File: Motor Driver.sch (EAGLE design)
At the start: 25 parts, among them U1 DRV8432_DKD_36, U2 LM27313

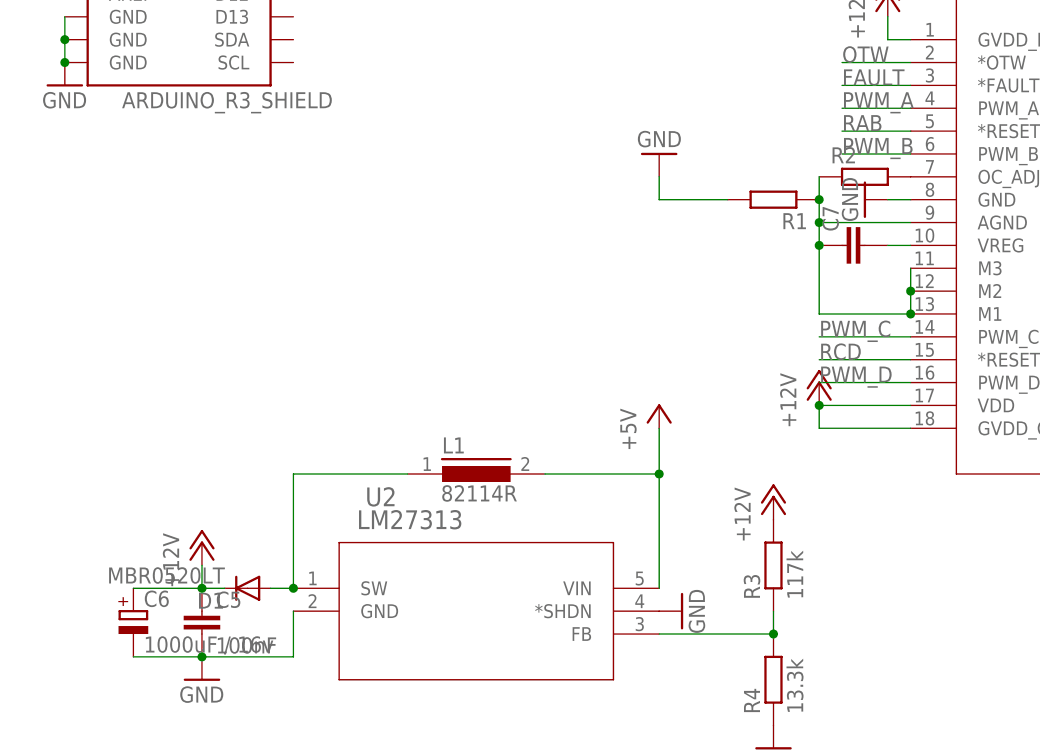
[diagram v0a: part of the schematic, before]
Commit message: Uploading Board
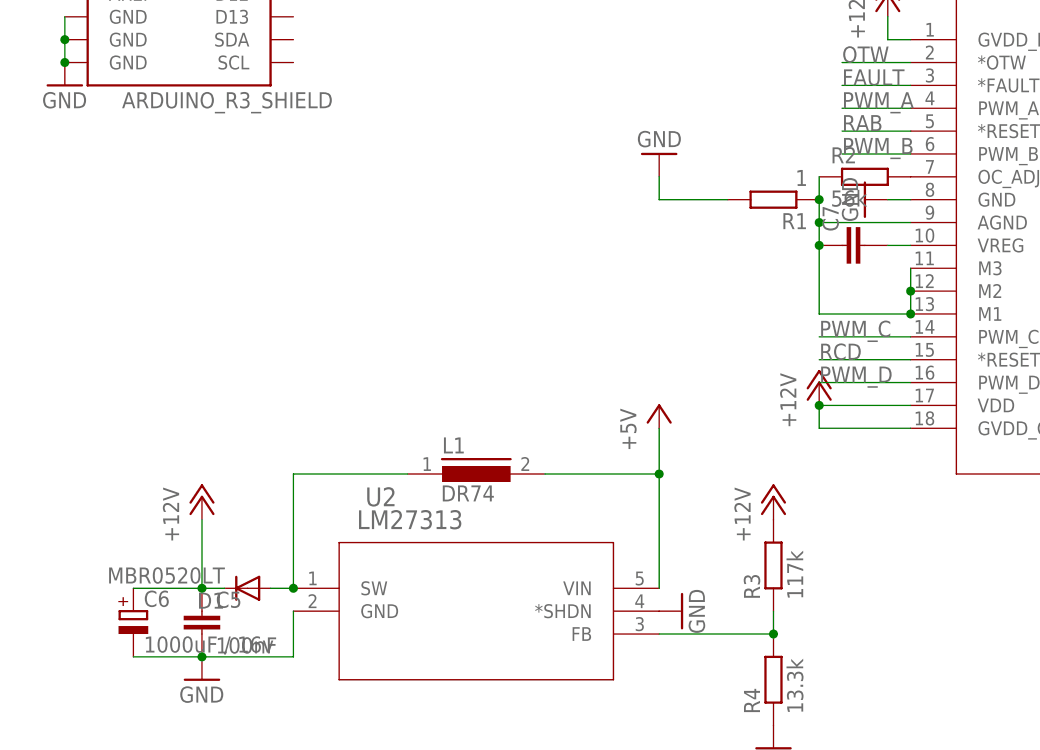
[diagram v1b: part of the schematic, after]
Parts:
- C1, C2, C3, C4: device resistor:C-EUC0805K -> resistor:C-EUC0402K
- L1: value 82114R -> DR74; device inductors:82114R -> inductors:DR74
- R1: value (none) -> 1
- R2: value (none) -> 56k
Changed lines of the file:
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@@
 <part name="U2" library="LM27313" deviceset="LM27313" device=""/>
 <part name="P+9" library="supply1" deviceset="+5V" device=""/>
-<part name="L1" library="inductors" deviceset="82114R" device=""/>
+<part name="L1" library="inductors" deviceset="DR74" device=""/>
 <part name="D1" library="diode" deviceset="MBR0520LT" device=""/>
 <part name="C5" library="resistor" deviceset="C-EU" device="C0805K" value="100nF"/>
@@
 <part name="P+10" library="supply1" deviceset="+12V" device=""/>
 <part name="P+11" library="supply1" deviceset="+12V" device=""/>
-<part name="C1" library="resistor" deviceset="C-EU" device="C0805K"/>
-<part name="C2" library="resistor" deviceset="C-EU" device="C0805K"/>
-<part name="C3" library="resistor" deviceset="C-EU" device="C0805K"/>
-<part name="C4" library="resistor" deviceset="C-EU" device="C0805K"/>
+<part name="C1" library="resistor" deviceset="C-EU" device="C0402K"/>
+<part name="C2" library="resistor" deviceset="C-EU" device="C0402K"/>
+<part name="C3" library="resistor" deviceset="C-EU" device="C0402K"/>
+<part name="C4" library="resistor" deviceset="C-EU" device="C0402K"/>
 <part name="C7" library="resistor" deviceset="C-EU" device="C0805K"/>
 <part name="C8" library="resistor" deviceset="C-EU" device="C0805K" value="100nF"/>
@@
 <part name="C12" library="resistor" deviceset="C-EU" device="C0805K" value="10nF"/>
 <part name="C13" library="resistor" deviceset="C-EU" device="C0805K" value="10nF"/>
-<part name="R1" library="resistor" deviceset="R-EU_" device="M0805"/>
-<part name="R2" library="resistor" deviceset="R-EU_" device="M0805"/>
+<part name="R1" library="resistor" deviceset="R-EU_" device="M0805" value="1"/>
+<part name="R2" library="resistor" deviceset="R-EU_" device="M0805" value="56k"/>
 <part name="GND2" library="supply1" deviceset="GND" device=""/>
 <part name="P+12" library="supply1" deviceset="VCC" device=""/>
@@
 <instance part="U2" gate="A" x="-30.48" y="17.78"/>
 <instance part="P+9" gate="1" x="-10.16" y="40.64"/>
-<instance part="L1" gate="1" x="-30.48" y="33.02"/>
+<instance part="L1" gate="G$1" x="-30.48" y="33.02"/>
 <instance part="D1" gate="G$1" x="-55.88" y="20.32" rot="R180"/>
 <instance part="C5" gate="G$1" x="-60.96" y="17.78"/>
 <instance part="C6" gate="G$1" x="-68.58" y="17.78"/>
-<instance part="P+10" gate="1" x="-60.96" y="25.4"/>
+<instance part="P+10" gate="1" x="-60.96" y="30.48"/>
 <instance part="P+11" gate="1" x="2.54" y="30.48"/>
 <instance part="C1" gate="G$1" x="81.28" y="78.74" rot="R90"/>
@@
 <junction x="-60.96" y="20.32"/>
 <pinref part="P+10" gate="1" pin="+12V"/>
-<wire x1="-60.96" y1="22.86" x2="-60.96" y2="20.32" width="0.1524" layer="91"/>
+<wire x1="-60.96" y1="27.94" x2="-60.96" y2="20.32" width="0.1524" layer="91"/>
 </segment>
 <segment>
@@
 <net name="+5V" class="0">
 <segment>
-<pinref part="L1" gate="1" pin="2"/>
+<pinref part="L1" gate="G$1" pin="2"/>
 <pinref part="U2" gate="A" pin="VIN"/>
 <wire x1="-22.86" y1="33.02" x2="-10.16" y2="33.02" width="0.1524" layer="91"/>
@@
 <net name="N$10" class="0">
 <segment>
-<pinref part="L1" gate="1" pin="1"/>
+<pinref part="L1" gate="G$1" pin="1"/>
 <pinref part="U2" gate="A" pin="SW"/>
 <wire x1="-38.1" y1="33.02" x2="-50.8" y2="33.02" width="0.1524" layer="91"/>
